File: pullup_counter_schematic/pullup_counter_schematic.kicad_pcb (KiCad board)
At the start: 2 copper layers, 75 x 45 mm, 53 parts, among them J1 FOUR_WIRE_CONN, J2 READ_PORT, Q1 MMBT3904, Q2 MMBT3904, Q3 MMBT3904, Q4 MMBT3906, SW1 SW_Push, U1 LM358, U2 HT7333, U3 P25Q40H, U4 dual_sev_seg_display, U5 AT24C02, U6 STM32F031C6Tx, Y1 32.768KHz

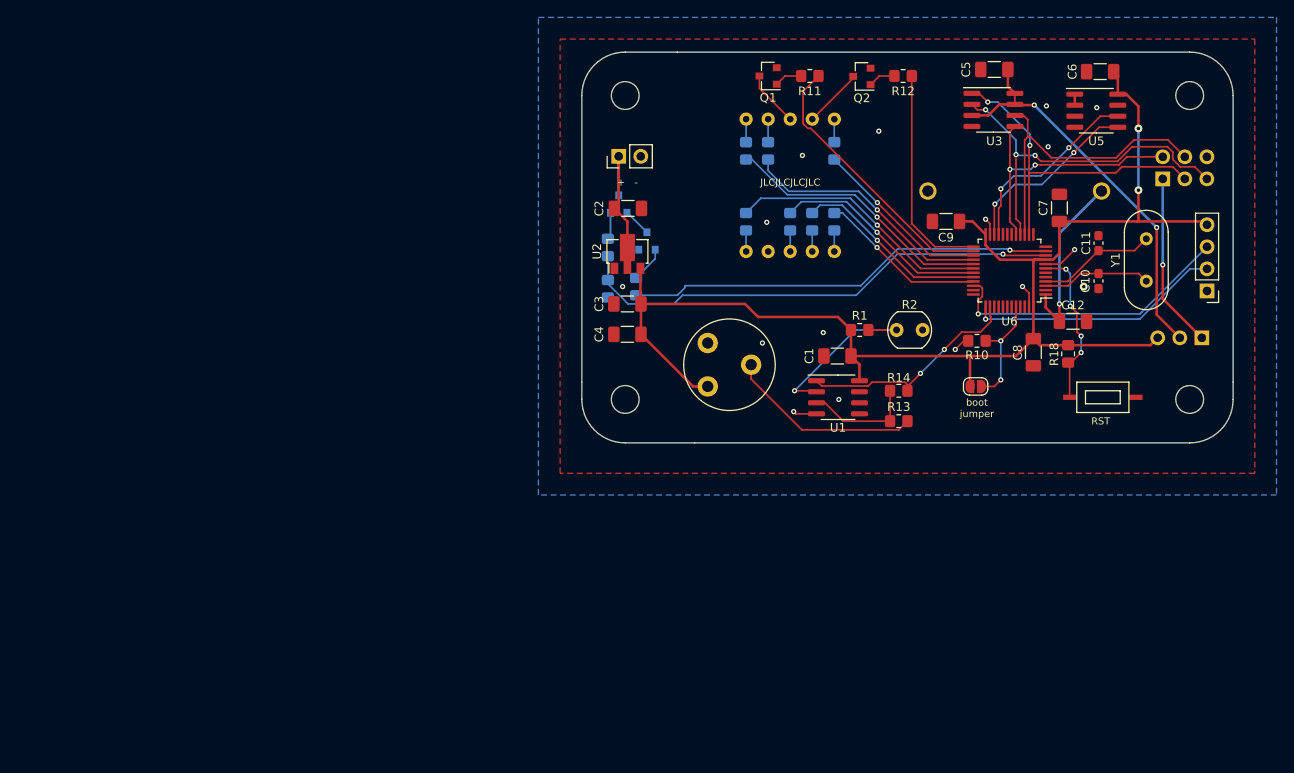
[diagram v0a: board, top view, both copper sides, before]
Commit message: Created PCB
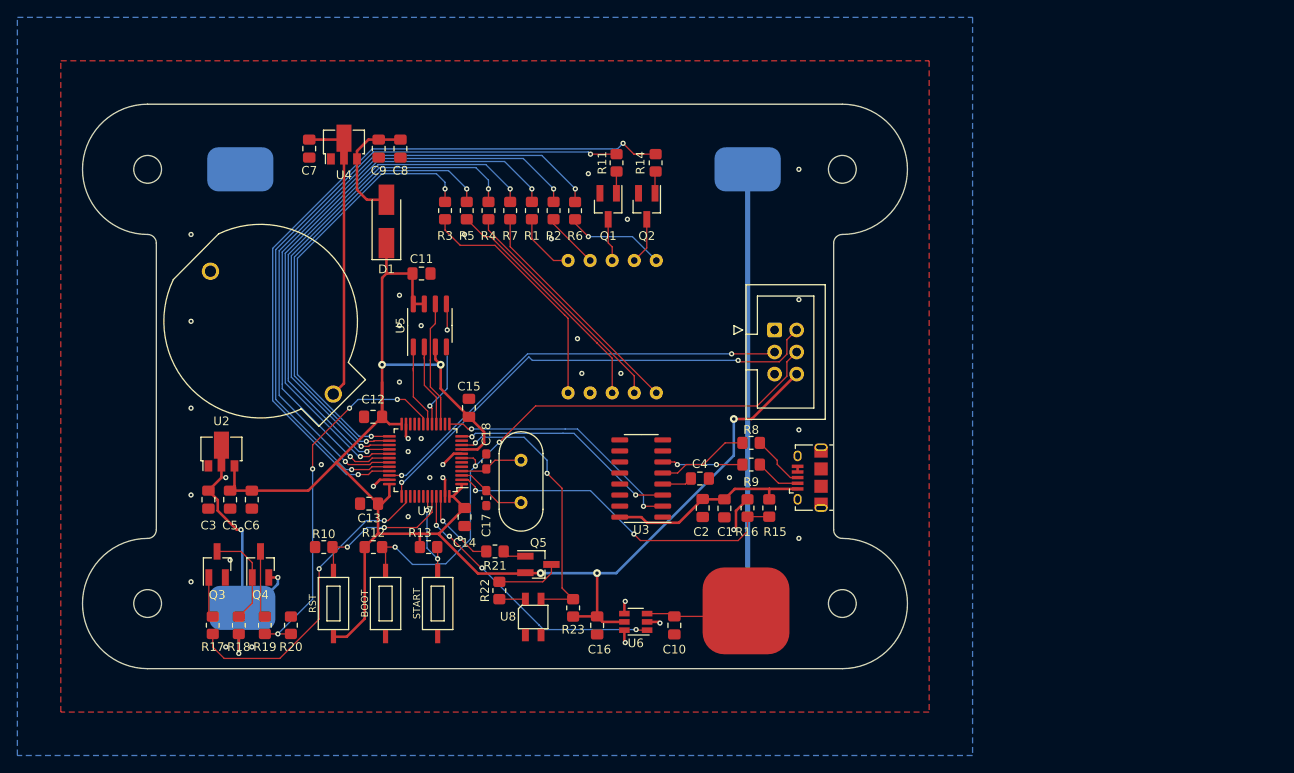
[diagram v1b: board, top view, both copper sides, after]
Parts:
- removed JP1: Jumper_2_Open, Jumper:SolderJumper-2_P1.3mm_Open_RoundedPad1.0x1.5mm
- removed JP2: Jumper_3_Open, Connector_PinSocket_2.54mm:PinSocket_1x03_P2.54mm_Vertical
- removed RN1: Voltage_Divider, Potentiometer_THT:Potentiometer_Piher_PT-10-V05_Vertical
- added BT3: CR2032, Battery_Custom:CR2032_CR2025_Battery_Holder, F.Cu at (113.0, 60.0)
- added C13: 100nF, Capacitor_SMD:C_0805_2012Metric_Pad1.18x1.45mm_HandSolder, F.Cu at (125.5, 81.0)
- added C14: 100nF, Capacitor_SMD:C_0805_2012Metric_Pad1.18x1.45mm_HandSolder, F.Cu at (136.5, 82.5)
- added C15: 4.7uF, Capacitor_SMD:C_0805_2012Metric_Pad1.18x1.45mm_HandSolder, F.Cu at (137.0, 70.0)
- added C16: 1uF, Capacitor_SMD:C_0805_2012Metric_Pad1.18x1.45mm_HandSolder, F.Cu at (151.8, 95.0)
- added C17: 10pF, Capacitor_SMD:C_0603_1608Metric_Pad1.08x0.95mm_HandSolder, F.Cu at (139.0, 80.4)
- added C18: 10pF, Capacitor_SMD:C_0603_1608Metric_Pad1.08x0.95mm_HandSolder, F.Cu at (139.0, 76.1)
- added D1: D_Schottky, Diode_SMD:D_SMA_Handsoldering, F.Cu at (127.5, 48.5)
- added Q5: MMBT3906, Package_TO_SOT_SMD:SOT-23_Handsoldering, F.Cu at (145.0, 88.0)
- added R19: 47K, Resistor_SMD:R_0805_2012Metric_Pad1.20x1.40mm_HandSolder, F.Cu at (113.5, 95.0)
- added R20: 47K, Resistor_SMD:R_0805_2012Metric_Pad1.20x1.40mm_HandSolder, F.Cu at (116.5, 95.0)
- added R21: R, Resistor_SMD:R_0805_2012Metric_Pad1.20x1.40mm_HandSolder, F.Cu at (140.0, 86.5)
- added R22: R, Resistor_SMD:R_0805_2012Metric_Pad1.20x1.40mm_HandSolder, F.Cu at (140.5, 91.0)
- added R23: R, Resistor_SMD:R_0805_2012Metric_Pad1.20x1.40mm_HandSolder, F.Cu at (149.0, 93.0)
- added SW2: rst, custom_buttons_switches:TSB008, F.Cu at (125.7, 89.5)
- added SW3: start, custom_buttons_switches:TSB008, F.Cu at (131.7, 89.5)
- added SW4: TouchPad, TouchPad:TouchPad_100x100, F.Cu at (168.9, 93.3)
- added U7: STM32L051C8Tx, Package_QFP:LQFP-48_7x7mm_P0.5mm, F.Cu at (132.0, 76.0)
- added U8: KTIR0711S, pullup_counter_schematic:KTIR0711S, F.Cu at (142.7, 95.4)
- BT1: value Battery -> LR03; footprint Connector_PinHeader_2.54mm:PinHeader_1x02_P2.54mm_Vertical -> Battery_Custom:SMD_SMT_AAA_LR03; moved to B.Cu
- BT2: value Battery_Cell -> LR03; footprint Battery_Custom:CR2032_CR2025_Battery_Holder -> Battery_Custom:SMD_SMT_AAA_LR03
- C1, C5: value 1uF -> 10uF; footprint Capacitor_SMD:C_1206_3216Metric_Pad1.33x1.80mm_HandSolder -> Capacitor_SMD:C_0805_2012Metric_Pad1.18x1.45mm_HandSolder
- C10: value 10pF -> ?pF; footprint Capacitor_SMD:C_0603_1608Metric_Pad1.08x0.95mm_HandSolder -> Capacitor_SMD:C_0805_2012Metric_Pad1.18x1.45mm_HandSolder
- C11: value 10pF -> 1uF; footprint Capacitor_SMD:C_0603_1608Metric_Pad1.08x0.95mm_HandSolder -> Capacitor_SMD:C_0805_2012Metric_Pad1.18x1.45mm_HandSolder
- C12, C3, C4: footprint Capacitor_SMD:C_1206_3216Metric_Pad1.33x1.80mm_HandSolder -> Capacitor_SMD:C_0805_2012Metric_Pad1.18x1.45mm_HandSolder
- C2: value 10uF -> 100nF; footprint Capacitor_SMD:C_1206_3216Metric_Pad1.33x1.80mm_HandSolder -> Capacitor_SMD:C_0805_2012Metric_Pad1.18x1.45mm_HandSolder
- C6: value 1uF -> 100nF; footprint Capacitor_SMD:C_1206_3216Metric_Pad1.33x1.80mm_HandSolder -> Capacitor_SMD:C_0805_2012Metric_Pad1.18x1.45mm_HandSolder
- C7, C8: value 100nF -> 10uF; footprint Capacitor_SMD:C_1206_3216Metric_Pad1.33x1.80mm_HandSolder -> Capacitor_SMD:C_0805_2012Metric_Pad1.18x1.45mm_HandSolder
- C9: value 4.7uF -> 100nF; footprint Capacitor_SMD:C_1206_3216Metric_Pad1.33x1.80mm_HandSolder -> Capacitor_SMD:C_0805_2012Metric_Pad1.18x1.45mm_HandSolder
- J1: value FOUR_WIRE_CONN -> USB_B_Micro; footprint Connector_PinHeader_2.54mm:PinHeader_1x04_P2.54mm_Vertical -> Connector_USB:USB_Micro-B_Amphenol_10118194_Horizontal
- J2: value READ_PORT -> 6PinDebugPort; footprint Connector_PinSocket_2.54mm:PinSocket_2x03_P2.54mm_Vertical -> Connector_IDC:IDC-Header_2x03_P2.54mm_Vertical; moved to F.Cu
- Q1, Q2: footprint Package_TO_SOT_SMD:SOT-23 -> Package_TO_SOT_SMD:SOT-23_Handsoldering
- Q3, Q4: footprint Package_TO_SOT_SMD:SOT-23 -> Package_TO_SOT_SMD:SOT-23_Handsoldering; moved to F.Cu
- R1: value 10K -> 1K
- R12: value 1K2 -> 10K
- R13: value R -> 10K
- R14: value R -> 1K2
- R15, R16, R17, R3, R4, R5, R6, R7: moved to F.Cu
- R18: value 10K -> 47K
- R2: value R_PHOTO -> 1K; footprint OptoDevice:R_LDR_5.0x4.1mm_P3mm_Vertical -> Resistor_SMD:R_0805_2012Metric_Pad1.20x1.40mm_HandSolder
- R8, R9: value 1K -> 220R; moved to F.Cu
- SW1: value SW_Push -> boot
- U1: value LM358 -> COM_C; footprint Package_SO:SOIC-8_3.9x4.9mm_P1.27mm -> Seven_Segment_Display_Custom:2_Digit_0_56_inch
- U2: value HT7333 -> HT7325
- U3: value P25Q40H -> CH340C; footprint Package_SO:SOIC-8_3.9x4.9mm_P1.27mm -> Package_SO:SOIC-16_3.9x9.9mm_P1.27mm
- U4: value dual_sev_seg_display -> HT7325; footprint Seven_Segment_Display_Custom:2_Digit_0_56_inch -> Package_TO_SOT_SMD:SOT-89-3
- U5: value AT24C02 -> P25Q40H
- U6: value STM32F031C6Tx -> TTP223; footprint Package_QFP:LQFP-48_7x7mm_P0.5mm -> Package_TO_SOT_SMD:TSOT-23-6
- moved H1 133.5 mm to (100.0, 92.5)
- moved C6 109.4 mm to (112.0, 80.5), turned to 270 degrees
- moved C5 101.0 mm to (109.5, 80.5), turned to 270 degrees
- moved R18 100.5 mm to (110.5, 95.0), turned to 90 degrees
- moved SW1 87.5 mm to (123.2, 95.5), turned to 90 degrees
- moved C7 86.7 mm to (118.6, 40.1), turned to 270 degrees
- moved R12 81.6 mm to (126.0, 86.0)
- moved C12 81.3 mm to (126.0, 71.0), turned to 180 degrees
- moved U5 80.6 mm to (132.5, 60.5), turned to 90 degrees
- moved R10 78.9 mm to (120.3, 86.0)
- moved C11 78.0 mm to (131.5, 54.5), turned to 0 degrees
- moved C8 76.6 mm to (129.1, 40.1)
- moved Y1 76.4 mm to (143.0, 80.9)
- moved BT1 68.9 mm to (109.0, 93.0), turned to 0 degrees
- moved C9 65.9 mm to (126.6, 40.1), turned to 270 degrees
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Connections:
- BT1 pad 2: GND -> Net-(BT1-Pad2)
- BT2 pad 1: +3V0 -> Net-(BT1-Pad2)
- C1 pad 1: +3V3 -> +5V
- C11 pad 1: Net-(C11-Pad1) -> VCC
- C12 pad 1: +3V0 -> VCC
- C2 pad 1: +BATT -> +5V
- C3 pad 1: +3V3 -> +BATT
- C4 pad 1: +3V3 -> Net-(C4-Pad1)
- C5 pad 1: /~HOLD -> VCC
- C6 pad 1: +3V3 -> VCC
- C7 pad 1: +3V3 -> +3V0
- C8 pad 1: +3V3 -> /V_BACKUP
- C9 pad 1: +3V3 -> /V_BACKUP
- J1 pad 1: GND -> +5V
- J1 pad 2: /SWCLK -> Net-(J1-Pad2)
- J1 pad 3: /SWDIO -> Net-(J1-Pad3)
- J1 pad 4: +3V3 -> GND
- J2 pad 1: /READ_PWR -> GND
- J2 pad 2: /MOSI -> /SWCLK
- J2 pad 3: /~CE -> /SWDIO
- J2 pad 4: /SCK -> /~RST
- J2 pad 5: /MISO -> (no net)
- J2 pad 6: GND -> VCC
- Q4 pad 2: Net-(Q4-Pad2) -> +BATT
- Q4 pad 3: +BATT -> Net-(Q4-Pad3)
- R1 pad 1: +3V3 -> Net-(R1-Pad1)
- R1 pad 2: /DIST_OUTA -> /dis_a
- R12 pad 1: Net-(Q2-Pad1) -> VCC
- R12 pad 2: /dis_sel_0 -> /~RST
- R13 pad 1: Net-(R13-Pad1) -> VCC
- R13 pad 2: /DIST_REF -> /Start
- R14 pad 1: /DIST_OUTD -> Net-(Q2-Pad1)
- R14 pad 2: Net-(R13-Pad1) -> /dis_sel_0
- R15 pad 1: Net-(Q3-Pad1) -> +5V
- R15 pad 2: /BAT_SENSE_EN -> /USB_FLAG
- R16 pad 1: /BAT_SENSE -> /USB_FLAG
- R16 pad 2: Net-(Q4-Pad2) -> GND
- R17 pad 1: GND -> Net-(Q3-Pad1)
- R17 pad 2: /BAT_SENSE -> /BAT_SENSE_EN
- R18 pad 1: +3V3 -> +BATT
- R18 pad 2: /~RST -> Net-(Q3-Pad3)
- R2 pad 1: /DIST_OUTA -> Net-(R2-Pad1)
- R2 pad 2: GND -> /dis_b
- R3 pad 2: /dis_a -> /dis_c
- R4 pad 2: /dis_b -> /dis_d
- R5 pad 2: /dis_c -> /dis_e
- R6 pad 2: /dis_d -> /dis_f
- R7 pad 2: /dis_e -> /dis_g
- R8 pad 1: Net-(R8-Pad1) -> Net-(J1-Pad3)
- R8 pad 2: /dis_f -> /USB_DP
- R9 pad 1: Net-(R9-Pad1) -> /USB_DM
- R9 pad 2: /dis_g -> Net-(J1-Pad2)
- SW1 pad 1: /~RST -> VCC
- SW1 pad 2: GND -> /boot
- U1 pad 1: /DIST_OUTD -> Net-(R3-Pad1)
- U1 pad 2: /DIST_OUTA -> (no net)
- U1 pad 3: Net-(R13-Pad1) -> Net-(R5-Pad1)
- U1 pad 4: GND -> Net-(R4-Pad1)
- U1 pad 5: GND -> Net-(R7-Pad1)
- U1 pad 6: GND -> Net-(R6-Pad1)
- U1 pad 7: (no net) -> /disp_pwr_0
- U1 pad 8: +3V3 -> /disp_pwr_1
- U2 pad 3: +3V3 -> VCC
- U3 pad 1: /~CE -> GND
- U3 pad 2: /MISO -> /MCU_RX
- U3 pad 3: /~HOLD -> /MCU_TX
- U3 pad 4: GND -> Net-(C4-Pad1)
- U3 pad 5: /MOSI -> /USB_DP
- U3 pad 6: /SCK -> /USB_DM
- U3 pad 7: /~HOLD -> (no net)
- U3 pad 8: /~HOLD -> (no net)
- U4 pad 1: Net-(R5-Pad1) -> GND
- U4 pad 2: (no net) -> +3V0
- U4 pad 3: Net-(R7-Pad1) -> /V_BACKUP
- U5 pad 1: GND -> /~CE
- U5 pad 2: GND -> /MISO
- U5 pad 3: GND -> VCC
- U5 pad 5: /SDA -> /MOSI
- U5 pad 6: /SCL -> /SCK
- U5 pad 7: GND -> VCC
- U5 pad 8: +3V3 -> VCC
- U6 pad 1: +3V0 -> /TouchPin
- U6 pad 2: (no net) -> GND
- U6 pad 4: Net-(C11-Pad1) -> GND
- U6 pad 5: (no net) -> VCC
- U6 pad 6: (no net) -> GND
- Y1 pad 1: Net-(C10-Pad1) -> Net-(C17-Pad1)
- Y1 pad 2: Net-(C11-Pad1) -> Net-(C18-Pad1)
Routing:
- net VCC: track 0.00 -> 193.1 mm, vias 0 -> 5
- net +3V3: track 154.5 -> 0.00 mm, vias 2 -> 0
- net /dis_sel_0: track 25.2 -> 84.3 mm, vias 0 -> 2
- net /dis_f: track 20.6 -> 74.5 mm, vias 1 -> 2
- net /~RST: track 18.7 -> 69.5 mm, vias 4 -> 3
- net Net-(BT1-Pad2): track 0.00 -> 50.6 mm
- net /~HOLD: track 46.2 -> 0.00 mm, vias 2 -> 0
- net /dis_sel_1: track 31.9 -> 77.8 mm, vias 0 -> 2
- net /dis_g: track 19.6 -> 62.2 mm, vias 1 -> 2
- net /dis_b: track 29.2 -> 70.4 mm, vias 1 -> 2
- net /USB_FLAG: track 0.00 -> 40.7 mm, vias 0 -> 2
- net /dis_d: track 22.4 -> 58.6 mm, vias 1 -> 2
- net /dis_a: track 31.2 -> 66.1 mm, vias 1 -> 2
- net /MISO: track 42.9 -> 9.69 mm, vias 3 -> 0
- net /TouchPin: track 0.00 -> 32.7 mm, vias 0 -> 4
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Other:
- board size 75 x 45 mm -> 95 x 65 mm
- board text added: "BOOT"
- board text added: "Otwory M3"
- board text added: "START"
- board text removed: "+ -"
- board text removed: "Debug Port"
- board text removed: "Flash Read Port"
- board text removed: "GND"
- board text removed: "JLCJLCJLCJLC"
- board text removed: "MOSI/SCK/GND VCC/~CE~/MISO"
- board text removed: "Normal Operation"
- board text removed: "Pull-up Counter - v01 - by Mkrysz"
- board text removed: "Read Data"
- board text removed: "SWCLK"
- board text removed: "SWDIO"
- board text removed: "VCC"
- board text removed: "boot jumper"
